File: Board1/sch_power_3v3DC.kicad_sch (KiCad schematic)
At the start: 6 parts, among them U2 TLV76133DCY

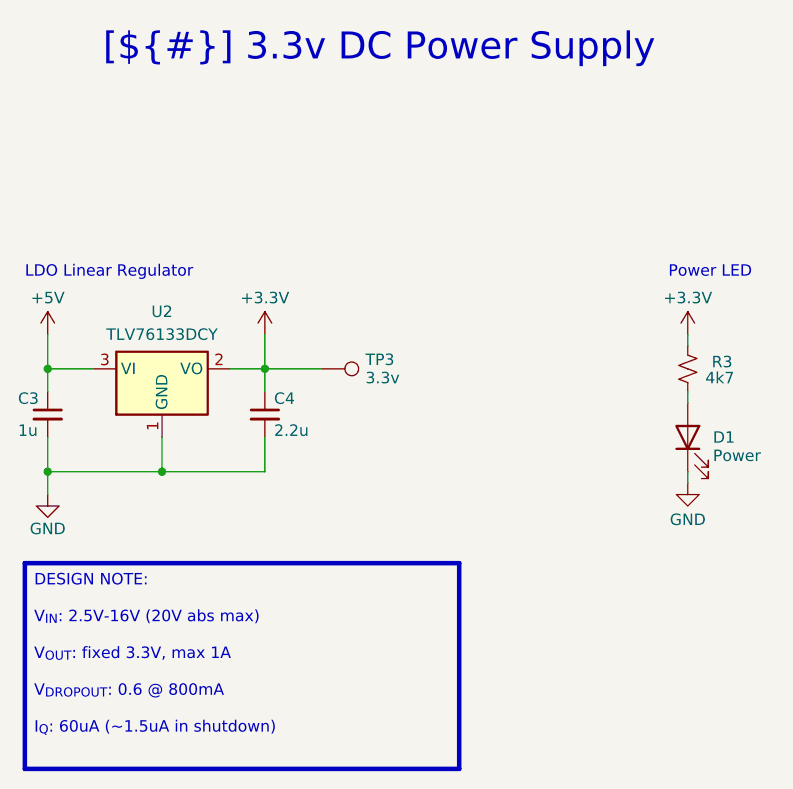
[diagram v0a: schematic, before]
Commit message: v1.2 release of board with bug fixes etc
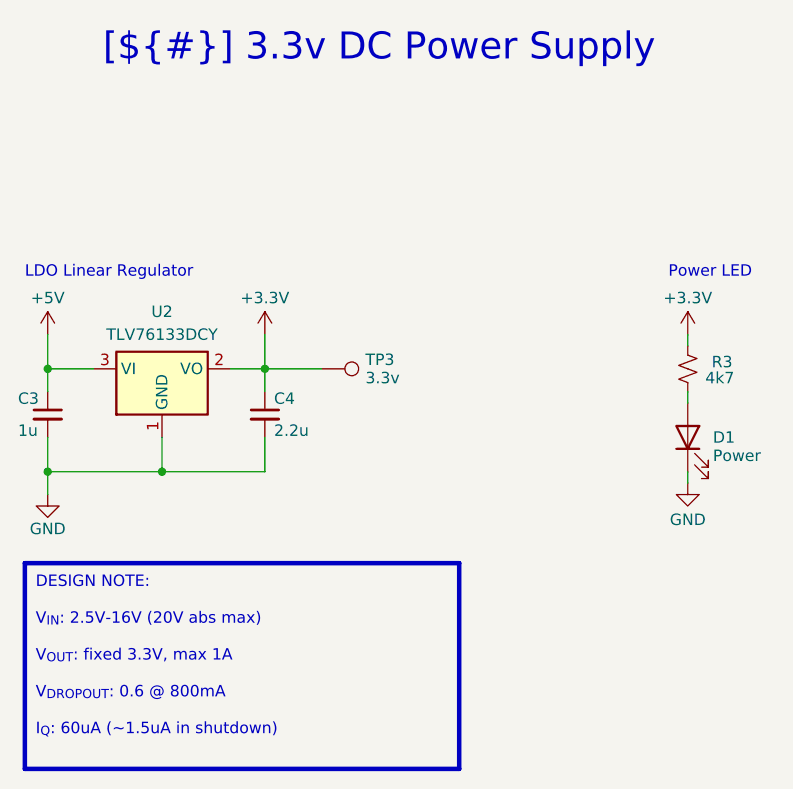
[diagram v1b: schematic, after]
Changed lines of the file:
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@@
 (kicad_sch
-	(version 20231120)
+	(version 20250114)
 	(generator "eeschema")
-	(generator_version "8.0")
+	(generator_version "9.0")
 	(paper "A4")
 	(title_block
 		(title "3.3v DC Power Supply")
-		(date "2025-02-19")
-		(rev "1.1")
+		(date "2025-03-08")
+		(rev "1.2")
 		(company "Wattle Labs")
 	)
-	(junction
-		(at 124.46 66.04)
-		(diameter 0)
-		(color 0 0 0 0)
-	)
-	(junction
-		(at 135.89 54.61)
-		(diameter 0)
-		(color 0 0 0 0)
-	)
-	(junction
-		(at 111.76 54.61)
-		(diameter 0)
-		(color 0 0 0 0)
-	)
-	(junction
-		(at 111.76 66.04)
-		(diameter 0)
-		(color 0 0 0 0)
-	)
-	(wire
-		(pts
-			(xy 124.46 66.04) (xy 135.89 66.04)
-		)
-		(stroke
-			(width 0)
-			(type default)
-		)
-	)
-	(wire
-		(pts
-			(xy 182.88 57.15) (xy 182.88 58.42)
-		)
-		(stroke
-			(width 0)
-			(type default)
-		)
-	)
-	(wire
-		(pts
-			(xy 124.46 66.04) (xy 124.46 62.23)
-		)
-		(stroke
-			(width 0)
-			(type default)
-		)
-	)
-	(wire
-		(pts
-			(xy 135.89 54.61) (xy 132.08 54.61)
-		)
-		(stroke
-			(width 0)
-			(type default)
-		)
-	)
-	(wire
-		(pts
-			(xy 111.76 50.8) (xy 111.76 54.61)
-		)
-		(stroke
-			(width 0)
-			(type default)
-		)
-	)
-	(wire
-		(pts
-			(xy 135.89 54.61) (xy 135.89 57.15)
-		)
-		(stroke
-			(width 0)
-			(type default)
-		)
-	)
-	(wire
-		(pts
-			(xy 182.88 50.8) (xy 182.88 52.07)
-		)
-		(stroke
-			(width 0)
-			(type default)
-		)
-	)
-	(wire
-		(pts
-			(xy 135.89 62.23) (xy 135.89 66.04)
-		)
-		(stroke
-			(width 0)
-			(type default)
-		)
-	)
-	(wire
-		(pts
-			(xy 111.76 54.61) (xy 116.84 54.61)
-		)
-		(stroke
-			(width 0)
-			(type default)
-		)
-	)
-	(wire
-		(pts
-			(xy 135.89 54.61) (xy 142.24 54.61)
-		)
-		(stroke
-			(width 0)
-			(type default)
-		)
-	)
-	(wire
-		(pts
-			(xy 111.76 66.04) (xy 124.46 66.04)
-		)
-		(stroke
-			(width 0)
-			(type default)
-		)
-	)
-	(wire
-		(pts
-			(xy 182.88 66.04) (xy 182.88 67.31)
-		)
-		(stroke
-			(width 0)
-			(type default)
-		)
-	)
-	(wire
-		(pts
-			(xy 135.89 50.8) (xy 135.89 54.61)
-		)
-		(stroke
-			(width 0)
-			(type default)
-		)
-	)
-	(wire
-		(pts
-			(xy 111.76 62.23) (xy 111.76 66.04)
-		)
-		(stroke
-			(width 0)
-			(type default)
-		)
-	)
-	(wire
-		(pts
-			(xy 111.76 66.04) (xy 111.76 68.58)
-		)
-		(stroke
-			(width 0)
-			(type default)
-		)
-	)
-	(wire
-		(pts
-			(xy 111.76 54.61) (xy 111.76 57.15)
-		)
-		(stroke
-			(width 0)
-			(type default)
+	(text "LDO Linear Regulator"
+		(exclude_from_sim no)
+		(at 109.22 43.18 0)
+		(effects
+			(font
+				(size 1.27 1.27)
+				(thickness 0.1588)
+			)
+			(justify left top)
+		)
+	)
+	(text "Power LED"
+		(exclude_from_sim no)
+		(at 180.721 43.18 0)
+		(effects
+			(font
+				(size 1.27 1.27)
+				(thickness 0.1588)
+			)
+			(justify left top)
 		)
 	)
@@
 		(at 109.22 76.2 0)
 		(size 48.26 22.86)
+		(margins 1.2025 1.2025 1.2025 1.2025)
 		(stroke
 			(width 0.5)
@@
 		(at 12.065 12.065 0)
 		(size 273.05 13.335)
+		(margins 2.2499 2.2499 2.2499 2.2499)
 		(stroke
 			(width -0.0001)
@@
 		)
 	)
-	(text "LDO Linear Regulator"
-		(exclude_from_sim no)
-		(at 109.22 43.18 0)
-		(effects
-			(font
-				(size 1.27 1.27)
-				(thickness 0.1588)
-			)
-			(justify left top)
-		)
-	)
-	(text "Power LED"
-		(exclude_from_sim no)
-		(at 180.721 43.18 0)
-		(effects
-			(font
-				(size 1.27 1.27)
-				(thickness 0.1588)
-			)
-			(justify left top)
-		)
-	)
+	(junction
+		(at 124.46 66.04)
+		(diameter 0)
+		(color 0 0 0 0)
+	)
+	(junction
+		(at 135.89 54.61)
+		(diameter 0)
+		(color 0 0 0 0)
+	)
+	(junction
+		(at 111.76 54.61)
+		(diameter 0)
+		(color 0 0 0 0)
+	)
+	(junction
+		(at 111.76 66.04)
+		(diameter 0)
+		(color 0 0 0 0)
+	)
+	(wire
+		(pts
+			(xy 124.46 66.04) (xy 135.89 66.04)
+		)
+		(stroke
+			(width 0)
+			(type default)
+		)
+	)
+	(wire
+		(pts
+			(xy 182.88 57.15) (xy 182.88 58.42)
+		)
+		(stroke
+			(width 0)
+			(type default)
+		)
+	)
+	(wire
+		(pts
+			(xy 124.46 66.04) (xy 124.46 62.23)
+		)
+		(stroke
+			(width 0)
+			(type default)
+		)
+	)
+	(wire
+		(pts
+			(xy 135.89 54.61) (xy 132.08 54.61)
+		)
+		(stroke
+			(width 0)
+			(type default)
+		)
+	)
+	(wire
+		(pts
+			(xy 111.76 50.8) (xy 111.76 54.61)
+		)
+		(stroke
+			(width 0)
+			(type default)
+		)
+	)
+	(wire
+		(pts
+			(xy 135.89 54.61) (xy 135.89 57.15)
+		)
+		(stroke
+			(width 0)
+			(type default)
+		)
+	)
+	(wire
+		(pts
+			(xy 182.88 50.8) (xy 182.88 52.07)
+		)
+		(stroke
+			(width 0)
+			(type default)
+		)
+	)
+	(wire
+		(pts
+			(xy 135.89 62.23) (xy 135.89 66.04)
+		)
+		(stroke
+			(width 0)
+			(type default)
+		)
+	)
+	(wire
+		(pts
+			(xy 111.76 54.61) (xy 116.84 54.61)
+		)
+		(stroke
+			(width 0)
+			(type default)
+		)
+	)
+	(wire
+		(pts
+			(xy 135.89 54.61) (xy 142.24 54.61)
+		)
+		(stroke
+			(width 0)
+			(type default)
+		)
+	)
+	(wire
+		(pts
+			(xy 111.76 66.04) (xy 124.46 66.04)
+		)
+		(stroke
+			(width 0)
+			(type default)
+		)
+	)
+	(wire
+		(pts
+			(xy 182.88 66.04) (xy 182.88 67.31)
+		)
+		(stroke
+			(width 0)
+			(type default)
+		)
+	)
+	(wire
+		(pts
+			(xy 135.89 50.8) (xy 135.89 54.61)
+		)
+		(stroke
+			(width 0)
+			(type default)
+		)
+	)
+	(wire
+		(pts
+			(xy 111.76 62.23) (xy 111.76 66.04)
+		)
+		(stroke
+			(width 0)
+			(type default)
+		)
+	)
+	(wire
+		(pts
+			(xy 111.76 66.04) (xy 111.76 68.58)
+		)
+		(stroke
+			(width 0)
+			(type default)
+		)
+	)
+	(wire
+		(pts
+			(xy 111.76 54.61) (xy 111.76 57.15)
+		)
+		(stroke
+			(width 0)
+			(type default)
+		)
+	)
